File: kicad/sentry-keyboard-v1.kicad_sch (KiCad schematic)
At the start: 269 parts, among them J2 Conn_01x04, J4 AVR-ISP-6, SW1 Reset, SW2 RotaryEncoder_Switch, U1 ATmega32U4-AU, Y1 16Mhz

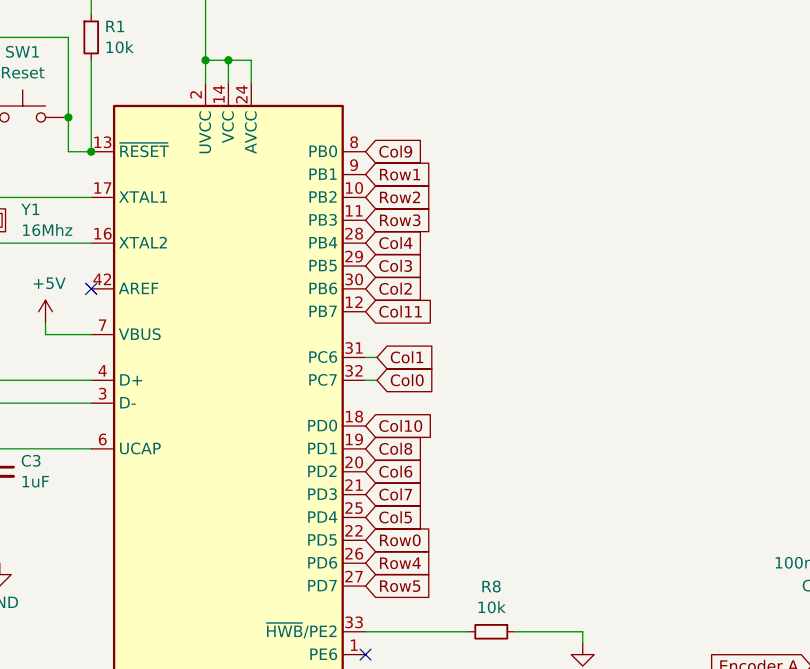
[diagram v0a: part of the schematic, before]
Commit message: Rough routing is complete
Still lots of small tweaks and clean up to do.
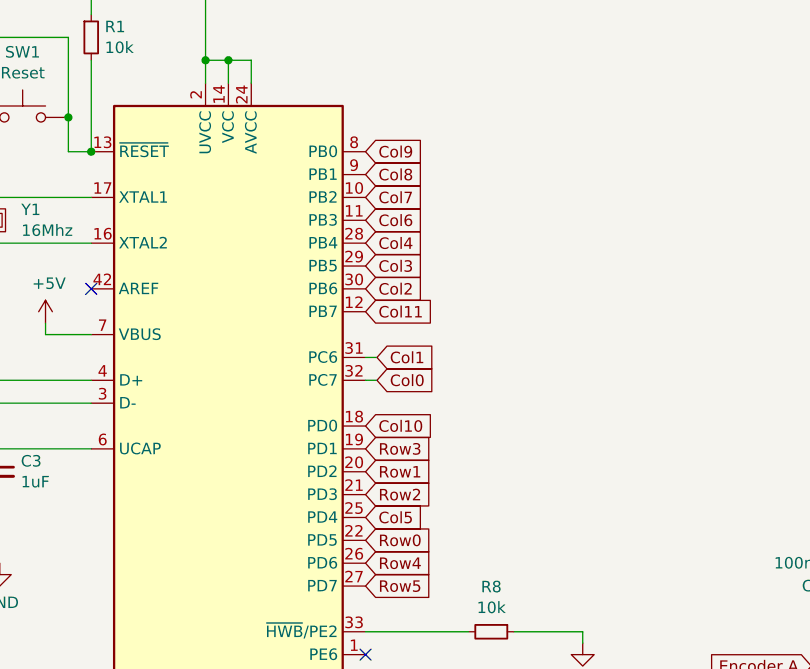
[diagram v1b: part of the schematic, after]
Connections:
- net Col6: now also U1.11 (PB3); no longer U1.20 (PD2)
- net Col7: now also U1.10 (PB2); no longer U1.21 (PD3)
- net Col8: now also U1.9 (PB1); no longer U1.19 (PD1)
- net Row1: now also U1.20 (PD2); no longer U1.9 (PB1)
- net Row2: now also U1.21 (PD3); no longer U1.10 (PB2)
- net Row3: now also U1.19 (PD1); no longer U1.11 (PB3)
